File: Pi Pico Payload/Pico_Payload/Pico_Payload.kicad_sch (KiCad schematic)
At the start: 9 parts, among them J1 ESC_2, J2 ESC_1, J3 Power_In, J4 Raspberry_Pi_4, U1 RaspberryPi_Pico

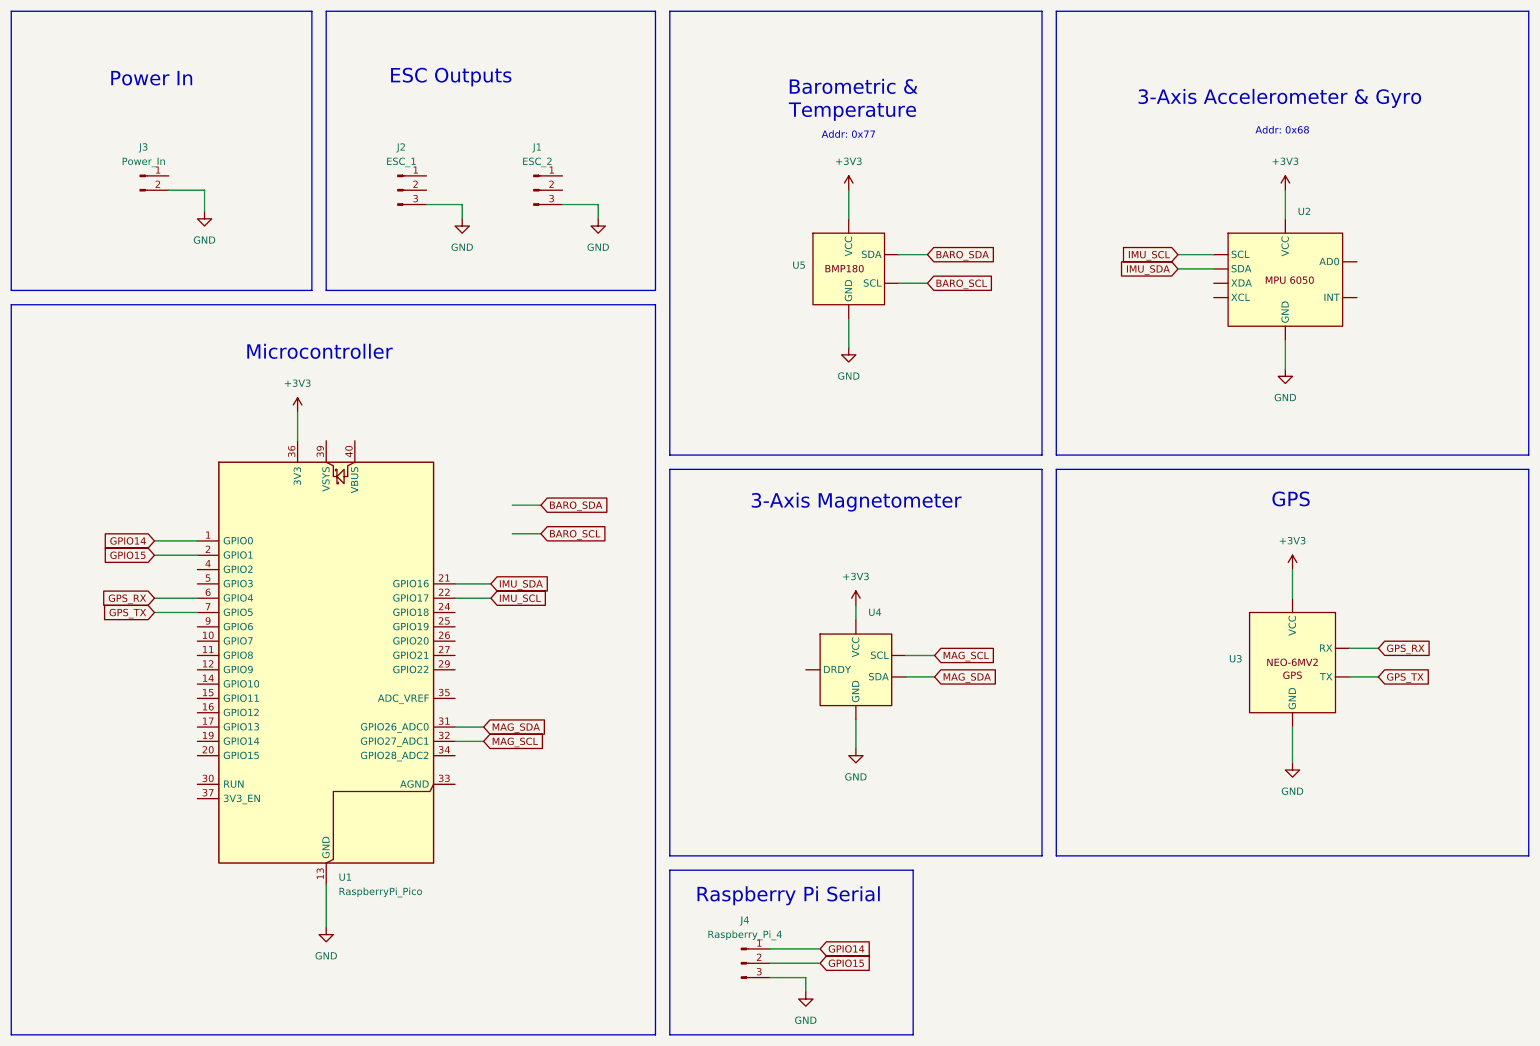
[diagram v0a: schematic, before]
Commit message: updated
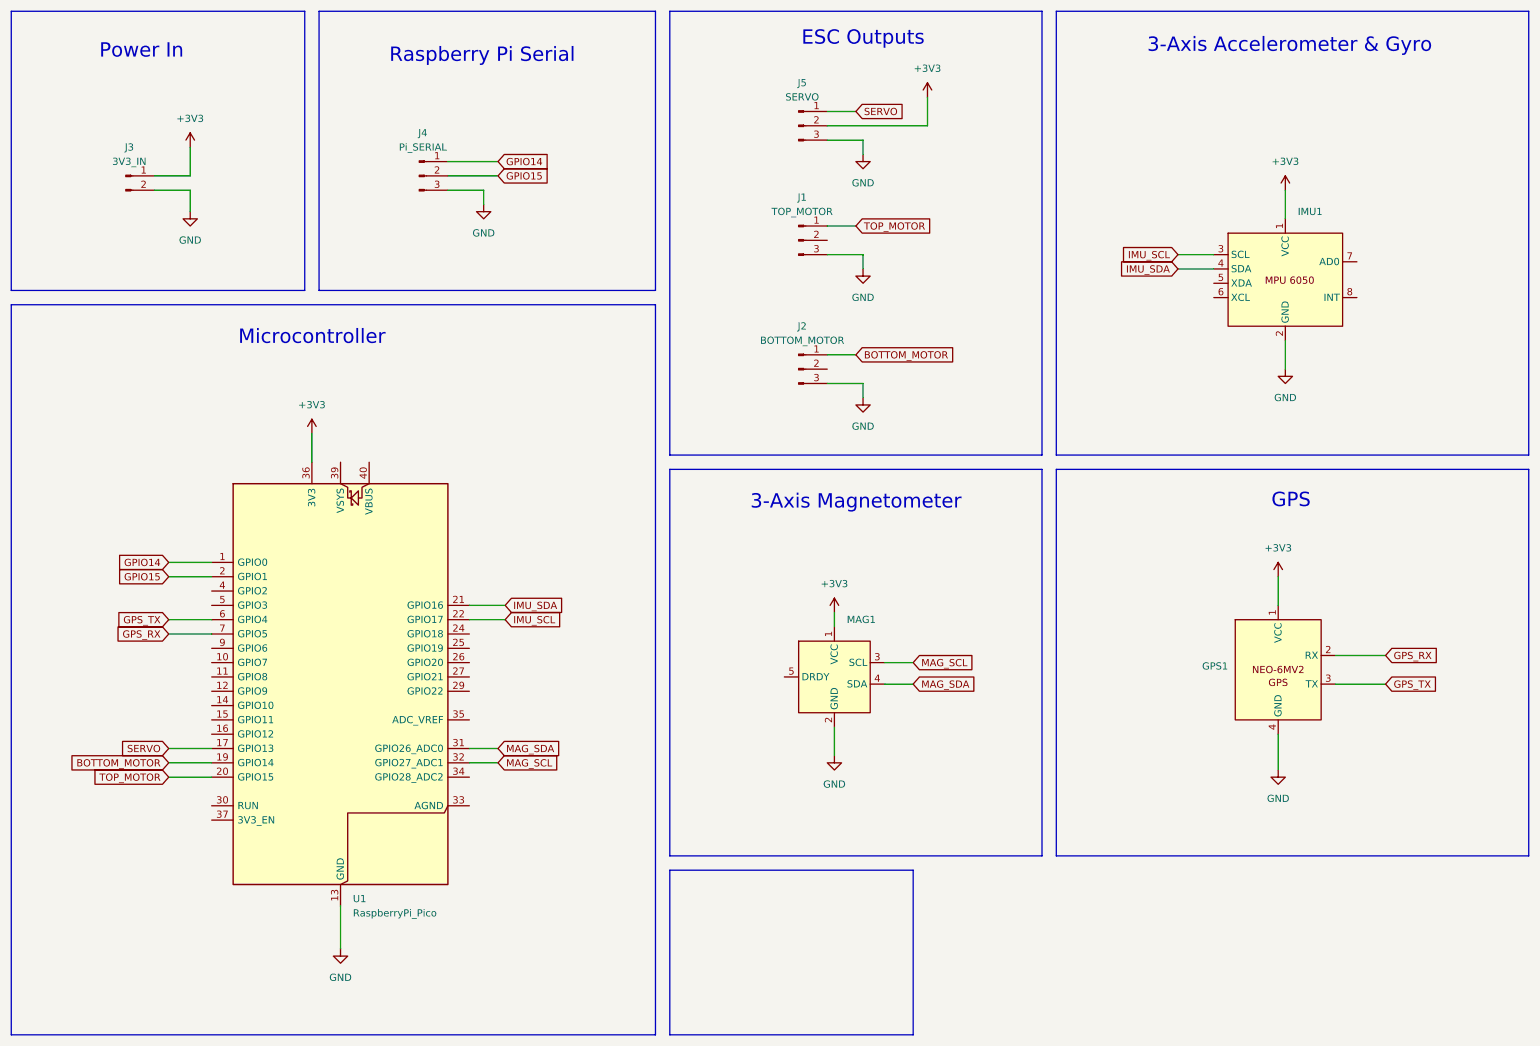
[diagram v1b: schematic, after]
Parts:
- removed U5: ~, symbol BMP180-Barometric-Sensor:BMP180
- added J5: SERVO, Connector_PinHeader_1.27mm:PinHeader_1x03_P1.27mm_Vertical, symbol Connector:Conn_01x03_Pin
- GPS1: renamed from U3; footprint (none) -> Connector_PinHeader_1.27mm:PinHeader_1x04_P1.27mm_Vertical
- IMU1: renamed from U2; footprint (none) -> Connector_PinHeader_1.27mm:PinHeader_1x08_P1.27mm_Vertical
- J1: value ESC_2 -> TOP_MOTOR; footprint (none) -> Connector_PinHeader_1.27mm:PinHeader_1x03_P1.27mm_Vertical
- J2: value ESC_1 -> BOTTOM_MOTOR; footprint (none) -> Connector_PinHeader_1.27mm:PinHeader_1x03_P1.27mm_Vertical
- J3: value Power_In -> 3V3_IN; footprint (none) -> Connector_PinHeader_1.27mm:PinHeader_1x02_P1.27mm_Vertical
- J4: value Raspberry_Pi_4 -> Pi_SERIAL; footprint (none) -> Connector_PinHeader_1.27mm:PinHeader_1x03_P1.27mm_Vertical
- MAG1: renamed from U4; footprint (none) -> Connector_PinHeader_1.27mm:PinHeader_1x05_P1.27mm_Vertical
- U1: footprint Module_RaspberryPi_Pico:RaspberryPi_Pico_Common -> Module_RaspberryPi_Pico:RaspberryPi_Pico_Original_SMD_MountingHoles_Castellated_HandSolder
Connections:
- net +3V3: now also GPS1.1 (VCC), IMU1.1 (VCC), J3.1 (Pin_1), MAG1.1 (VCC), J5.2 (Pin_2); no longer GPS1. (VCC), IMU1. (XDA), MAG1. (VCC)
- net GND: now also GPS1.4 (GND), IMU1.2 (GND), MAG1.2 (GND), J5.3 (Pin_3); no longer GPS1. (VCC), IMU1. (XDA), MAG1. (VCC)
- net GPS_RX: now also GPS1.2 (RX), U1.7 (GPIO5); no longer GPS1. (VCC), U1.6 (GPIO4)
- net GPS_TX: now also GPS1.3 (TX), U1.6 (GPIO4); no longer GPS1. (VCC), U1.7 (GPIO5)
- net IMU_SCL: now also IMU1.3 (SCL); no longer IMU1. (XDA)
- net IMU_SDA: now also IMU1.4 (SDA); no longer IMU1. (XDA)
- net MAG_SCL: now also MAG1.3 (SCL); no longer MAG1. (VCC)
- net MAG_SDA: now also MAG1.4 (SDA); no longer MAG1. (VCC)
- net BOTTOM_MOTOR: now reaches J2.1 (Pin_1)
- net BOTTOM_MOTOR: now also U1.19 (GPIO14)
- net TOP_MOTOR: now reaches J1.1 (Pin_1)
- net TOP_MOTOR: now also U1.20 (GPIO15)
- net SERVO: now reaches U1.17 (GPIO13)
- net SERVO: now also J5.1 (Pin_1)
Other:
- note removed: "Addr: 0x68"
- note removed: "Addr: 0x77"
- note removed: "Barometric & Temperature"
- moved on the sheet: J3, U1

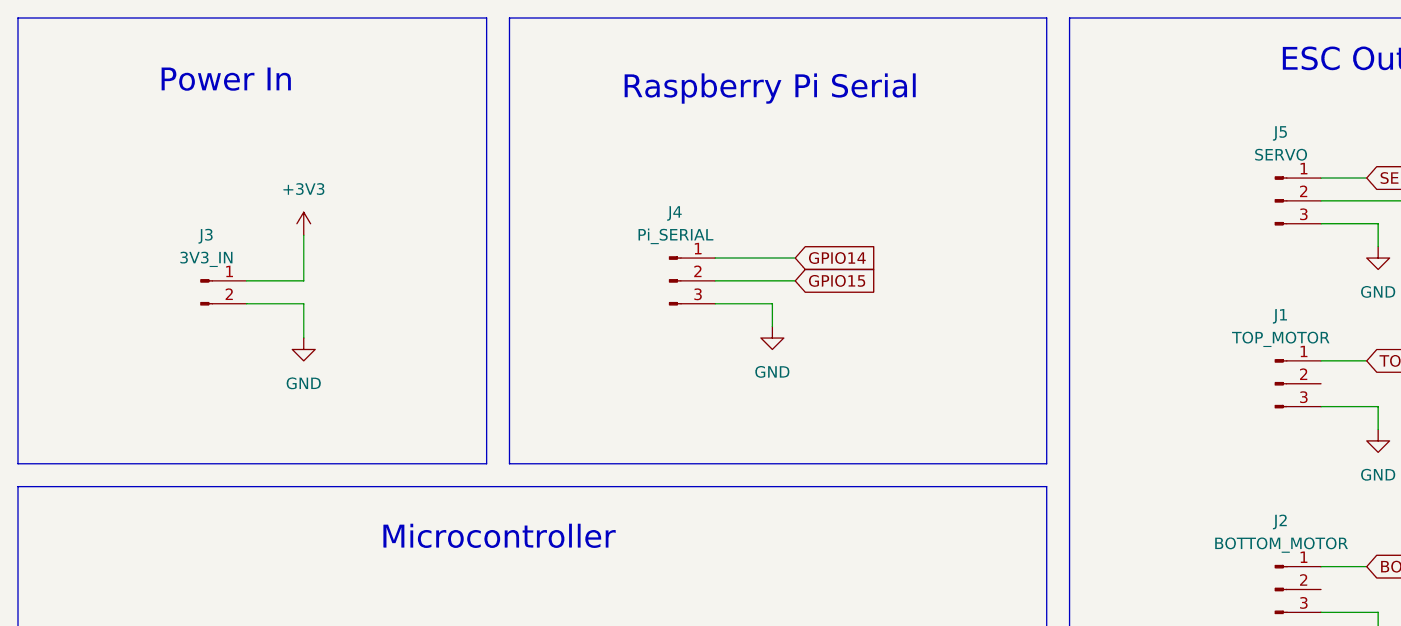
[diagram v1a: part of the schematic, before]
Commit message: updated
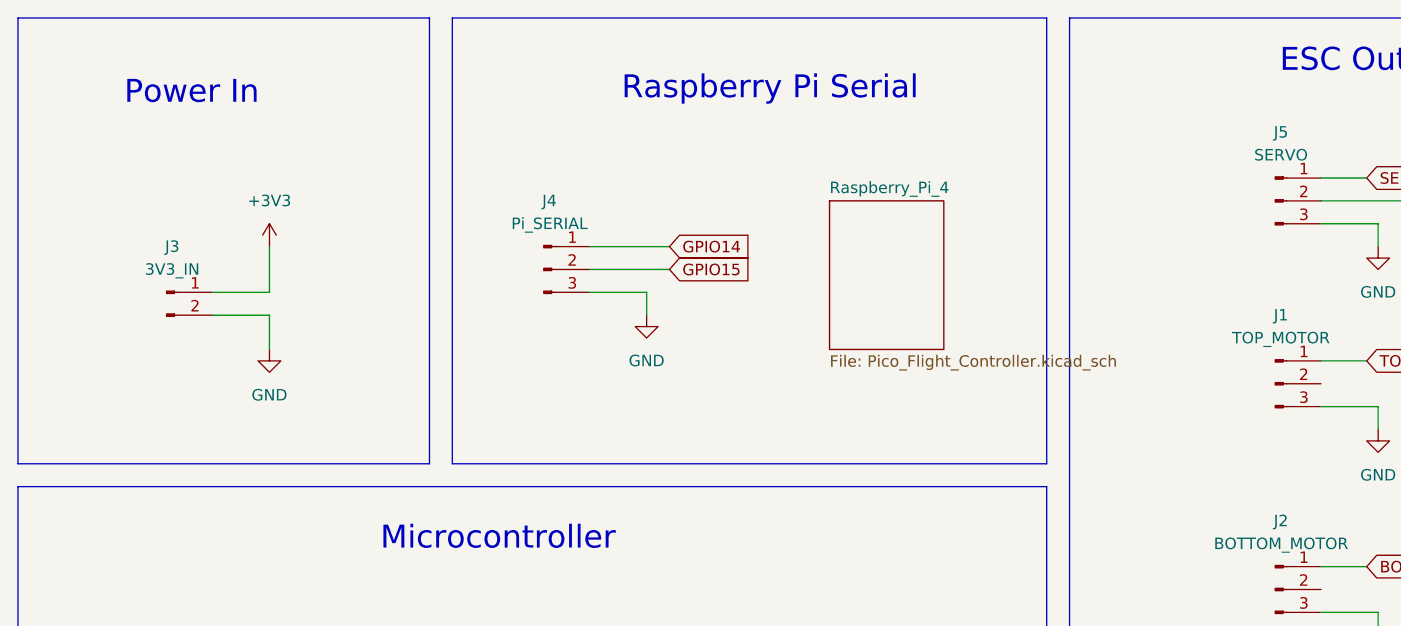
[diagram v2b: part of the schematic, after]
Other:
- added sheet Raspberry_Pi_4 (Pico_Flight_Controller.kicad_sch)
- moved on the sheet: J3, J4
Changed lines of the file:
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@@
 	(wire
 		(pts
-			(xy 91.44 45.72) (xy 97.79 45.72)
+			(xy 77.47 44.45) (xy 83.82 44.45)
 		)
 		(stroke
@@
 	(wire
 		(pts
-			(xy 91.44 40.64) (xy 100.33 40.64)
+			(xy 77.47 39.37) (xy 86.36 39.37)
 		)
 		(stroke
@@
 	(wire
 		(pts
-			(xy 39.37 43.18) (xy 45.72 43.18)
+			(xy 35.56 44.45) (xy 41.91 44.45)
 		)
 		(stroke
@@
 	(wire
 		(pts
-			(xy 39.37 45.72) (xy 45.72 45.72)
+			(xy 35.56 46.99) (xy 41.91 46.99)
 		)
 		(stroke
@@
 	(wire
 		(pts
-			(xy 97.79 45.72) (xy 97.79 48.26)
+			(xy 83.82 44.45) (xy 83.82 46.99)
 		)
 		(stroke
@@
 	(wire
 		(pts
-			(xy 45.72 45.72) (xy 45.72 49.53)
+			(xy 41.91 46.99) (xy 41.91 50.8)
 		)
 		(stroke
@@
 	(wire
 		(pts
-			(xy 91.44 43.18) (xy 100.33 43.18)
+			(xy 77.47 41.91) (xy 86.36 41.91)
 		)
 		(stroke
@@
 	(wire
 		(pts
-			(xy 45.72 38.1) (xy 45.72 43.18)
+			(xy 41.91 39.37) (xy 41.91 44.45)
 		)
 		(stroke
@@
 	(rectangle
 		(start 13.97 13.97)
-		(end 66.04 63.5)
+		(end 59.69 63.5)
 		(stroke
 			(width 0)
@@
 	)
 	(rectangle
-		(start 68.58 13.97)
+		(start 62.23 13.97)
 		(end 128.27 63.5)
 		(stroke
@@
 	(text "Power In"
 		(exclude_from_sim no)
-		(at 37.084 21.082 0)
+		(at 33.274 22.352 0)
 		(effects
 			(font
@@
 	(global_label "GPIO15"
 		(shape input)
-		(at 100.33 43.18 0)
+		(at 86.36 41.91 0)
 		(fields_autoplaced yes)
 		(effects
@@
 		)
 		(property "Intersheetrefs" "${INTERSHEET_REFS}"
-			(at 110.2095 43.18 0)
+			(at 96.2395 41.91 0)
 			(effects
 				(font
@@
 	(global_label "GPIO14"
 		(shape input)
-		(at 100.33 40.64 0)
+		(at 86.36 39.37 0)
 		(fields_autoplaced yes)
 		(effects
@@
 		)
 		(property "Intersheetrefs" "${INTERSHEET_REFS}"
-			(at 110.2095 40.64 0)
+			(at 96.2395 39.37 0)
 			(effects
 				(font
@@
 	(symbol
 		(lib_id "Connector:Conn_01x02_Pin")
-		(at 34.29 43.18 0)
+		(at 30.48 44.45 0)
 		(unit 1)
 		(exclude_from_sim no)
@@
 		(fields_autoplaced yes)
 		(property "Reference" "J3"
-			(at 34.925 38.1 0)
+			(at 31.115 39.37 0)
 			(effects
 				(font
@@
 		)
 		(property "Value" "3V3_IN"
-			(at 34.925 40.64 0)
+			(at 31.115 41.91 0)
 			(effects
 				(font
@@
 		)
 		(property "Footprint" "Connector_PinHeader_1.27mm:PinHeader_1x02_P1.27mm_Vertical"
-			(at 34.29 43.18 0)
+			(at 30.48 44.45 0)
 			(effects
 				(font
@@
 		)
 		(property "Datasheet" "~"
-			(at 34.29 43.18 0)
+			(at 30.48 44.45 0)
 			(effects
 				(font
@@
 		)
 		(property "Description" "Generic connector, single row, 01x02, script generated"
-			(at 34.29 43.18 0)
+			(at 30.48 44.45 0)
 			(effects
 				(font
@@
 	(symbol
 		(lib_id "power:GND")
-		(at 97.79 48.26 0)
+		(at 83.82 46.99 0)
 		(unit 1)
 		(exclude_from_sim no)
@@
 		(fields_autoplaced yes)
 		(property "Reference" "#PWR02"
-			(at 97.79 54.61 0)
+			(at 83.82 53.34 0)
 			(effects
 				(font
@@
 		)
 		(property "Value" "GND"
-			(at 97.79 53.34 0)
+			(at 83.82 52.07 0)
 			(effects
 				(font
@@
 		)
 		(property "Footprint" ""
-			(at 97.79 48.26 0)
+			(at 83.82 46.99 0)
 			(effects
 				(font
@@
 		)
 		(property "Datasheet" ""
-			(at 97.79 48.26 0)
+			(at 83.82 46.99 0)
 			(effects
 				(font
@@
 		)
 		(property "Description" "Power symbol creates a global label with name \"GND\" , ground"
-			(at 97.79 48.26 0)
+			(at 83.82 46.99 0)
 			(effects
 				(font
@@
 	(symbol
 		(lib_id "power:GND")
-		(at 45.72 49.53 0)
+		(at 41.91 50.8 0)
 		(unit 1)
 		(exclude_from_sim no)
@@
 		(fields_autoplaced yes)
 		(property "Reference" "#PWR06"
-			(at 45.72 55.88 0)
+			(at 41.91 57.15 0)
 			(effects
 				(font
@@
 		)
 		(property "Value" "GND"
-			(at 45.72 54.61 0)
+			(at 41.91 55.88 0)
 			(effects
 				(font
@@
 		)
 		(property "Footprint" ""
-			(at 45.72 49.53 0)
+			(at 41.91 50.8 0)
 			(effects
 				(font
@@
 		)
 		(property "Datasheet" ""
-			(at 45.72 49.53 0)
+			(at 41.91 50.8 0)
 			(effects
 				(font
@@
 		)
 		(property "Description" "Power symbol creates a global label with name \"GND\" , ground"
-			(at 45.72 49.53 0)
+			(at 41.91 50.8 0)
 			(effects
 				(font
@@
 	(symbol
 		(lib_id "Connector:Conn_01x03_Pin")
-		(at 86.36 43.18 0)
+		(at 72.39 41.91 0)
 		(unit 1)
 		(exclude_from_sim no)
@@
 		(fields_autoplaced yes)
 		(property "Reference" "J4"
-			(at 86.995 35.56 0)
+			(at 73.025 34.29 0)
 			(effects
 				(font
@@
 		)
 		(property "Value" "Pi_SERIAL"
-			(at 86.995 38.1 0)
+			(at 73.025 36.83 0)
 			(effects
 				(font
@@
 		)
 		(property "Footprint" "Connector_PinHeader_1.27mm:PinHeader_1x03_P1.27mm_Vertical"
-			(at 86.36 43.18 0)
+			(at 72.39 41.91 0)
 			(effects
 				(font
@@
 		)
 		(property "Datasheet" "~"
-			(at 86.36 43.18 0)
+			(at 72.39 41.91 0)
 			(effects
 				(font
@@
 		)
 		(property "Description" "Generic connector, single row, 01x03, script generated"
-			(at 86.36 43.18 0)
+			(at 72.39 41.91 0)
 			(effects
 				(font
@@
 	(symbol
 		(lib_id "power:+3V3")
-		(at 45.72 38.1 0)
+		(at 41.91 39.37 0)
 		(unit 1)
 		(exclude_from_sim no)
@@
 		(fields_autoplaced yes)
 		(property "Reference" "#PWR015"
-			(at 45.72 41.91 0)
+			(at 41.91 43.18 0)
 			(effects
 				(font
@@
 		)
 		(property "Value" "+3V3"
-			(at 45.72 33.02 0)
+			(at 41.91 34.29 0)
 			(effects
 				(font
@@
 		)
 		(property "Footprint" ""
-			(at 45.72 38.1 0)
+			(at 41.91 39.37 0)
 			(effects
 				(font
@@
 		)
 		(property "Datasheet" ""
-			(at 45.72 38.1 0)
+			(at 41.91 39.37 0)
 			(effects
 				(font
@@
 		)
 		(property "Description" "Power symbol creates a global label with name \"+3V3\""
-			(at 45.72 38.1 0)
+			(at 41.91 39.37 0)
 			(effects
 				(font
@@
 				)
 			)
+		)
+	)
+	(sheet
+		(at 104.14 34.29)
+		(size 12.7 16.51)
+		(fields_autoplaced yes)
+		(stroke
+			(width 0.1524)
+			(type solid)
+		)
+		(fill
+			(color 0 0 0 0.0000)
+		)
+		(property "Sheetname" "Raspberry_Pi_4"
+			(at 104.14 33.5784 0)
+			(effects
+				(font
+					(size 1.27 1.27)
+				)
+				(justify left bottom)
+			)
+		)
+		(property "Sheetfile" "Pico_Flight_Controller.kicad_sch"
+			(at 104.14 51.3846 0)
+			(effects
+				(font
+					(size 1.27 1.27)
+				)
+				(justify left top)
+			)
+		)
+		(instances
+			(project "Pico_Payload"
+				(path "/e35ac035-ac8e-47a6-8b34-6cf6678b8476"
+					(page "2")
+				)
+			)
